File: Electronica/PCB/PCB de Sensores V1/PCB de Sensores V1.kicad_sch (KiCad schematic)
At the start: 10 parts, among them J1 Conn_02x08_Odd_Even, J2 Conexion Sensores, U1 ULTRASONICO1, U2 ULTRASONICO2, U3 ULTRASONICO3, U4 ULTRASONICO4, U5 ULTRASONICO5

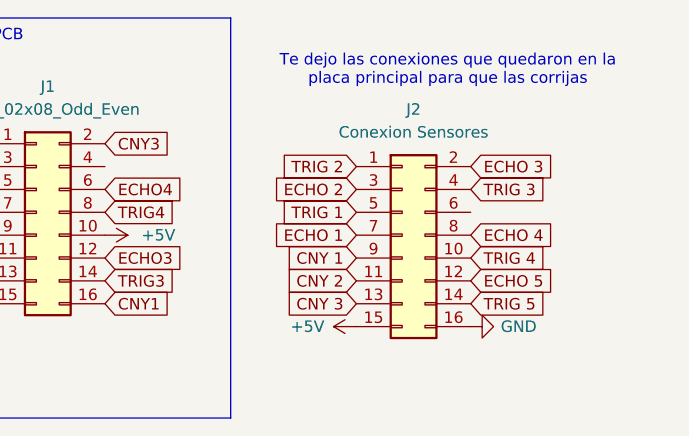
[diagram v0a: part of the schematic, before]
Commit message: SELIGRAFIA
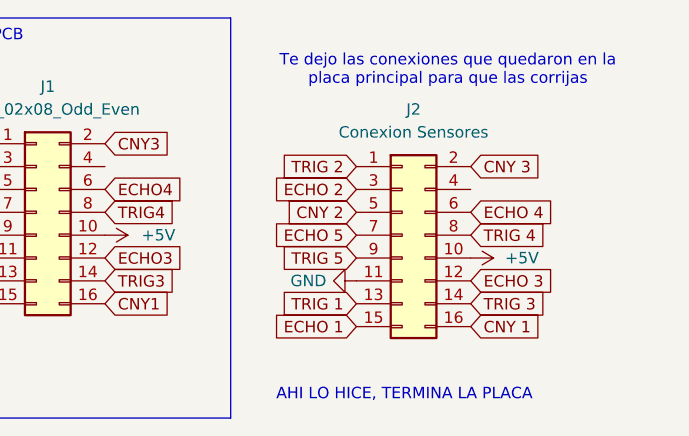
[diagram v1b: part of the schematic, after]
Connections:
- net +5V: now also J2.10 (Pin_10); no longer J2.15 (Pin_15)
- net CNY 1: now also J2.16 (Pin_16); no longer J2.9 (Pin_9)
- net CNY 2: now also J2.5 (Pin_5); no longer J2.11 (Pin_11)
- net CNY 3: now also J2.2 (Pin_2); no longer J2.13 (Pin_13)
- net ECHO 1: now also J2.15 (Pin_15); no longer J2.7 (Pin_7)
- net ECHO 3: now also J2.12 (Pin_12); no longer J2.2 (Pin_2)
- net ECHO 4: now also J2.6 (Pin_6); no longer J2.8 (Pin_8)
- net ECHO 5: now also J2.7 (Pin_7); no longer J2.12 (Pin_12)
- net GND: now also J2.11 (Pin_11); no longer J2.16 (Pin_16)
- net TRIG 1: now also J2.13 (Pin_13); no longer J2.5 (Pin_5)
- net TRIG 3: now also J2.14 (Pin_14); no longer J2.4 (Pin_4)
- net TRIG 4: now also J2.8 (Pin_8); no longer J2.10 (Pin_10)
- net TRIG 5: now also J2.9 (Pin_9); no longer J2.14 (Pin_14)
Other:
- note added: "AHI LO HICE, TERMINA LA PLACA"

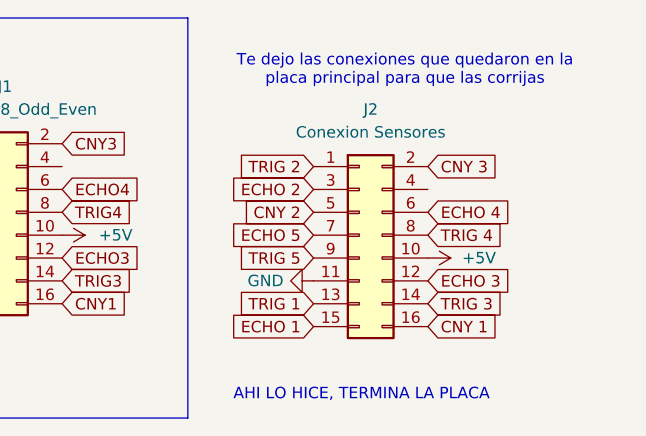
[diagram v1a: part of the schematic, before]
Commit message: Codigo nuevo sin terminar
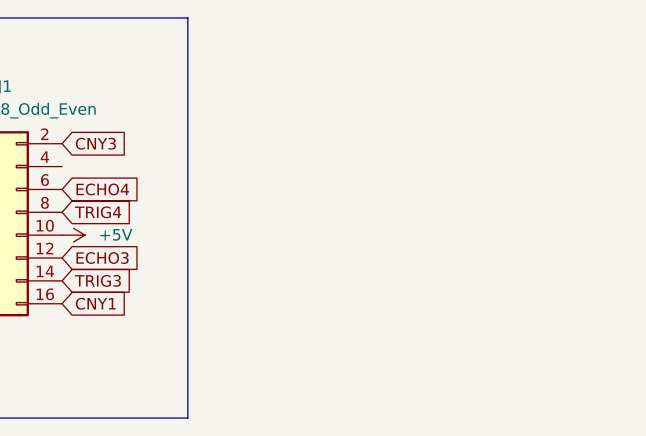
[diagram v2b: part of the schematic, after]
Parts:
- removed J2: Conexion Sensores, Connector_PinHeader_2.54mm:PinHeader_2x08_P2.54mm_Horizontal, symbol Connector_Generic:Conn_02x08_Odd_Even
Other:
- note removed: "AHI LO HICE, TERMINA LA PLACA"
- note removed: "Te dejo las conexiones que quedaron en la placa principal para que las corrijas"
